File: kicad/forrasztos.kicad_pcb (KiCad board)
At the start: 2 copper layers, 115 x 70.6 mm, 91 parts, among them J1 24V+-, J2 Conn_02x04_Pin, J3 Conn_01x20_Pin, J4 Conn_01x06_Pin, J5 Conn_02x04_Pin, Q1 AOD409, Q2 MMST2222A, Q3 AOD409, Q4 MMST2222A, SW1 RotaryEncoder_Switch, SW2 SW_Push, SW3 SW_Push, U1 AP63205WU, U2 MCP6004, U3 AP63203WU, U4 24LC00, U5 STM32F103C8Tx, Y1 ATS080B

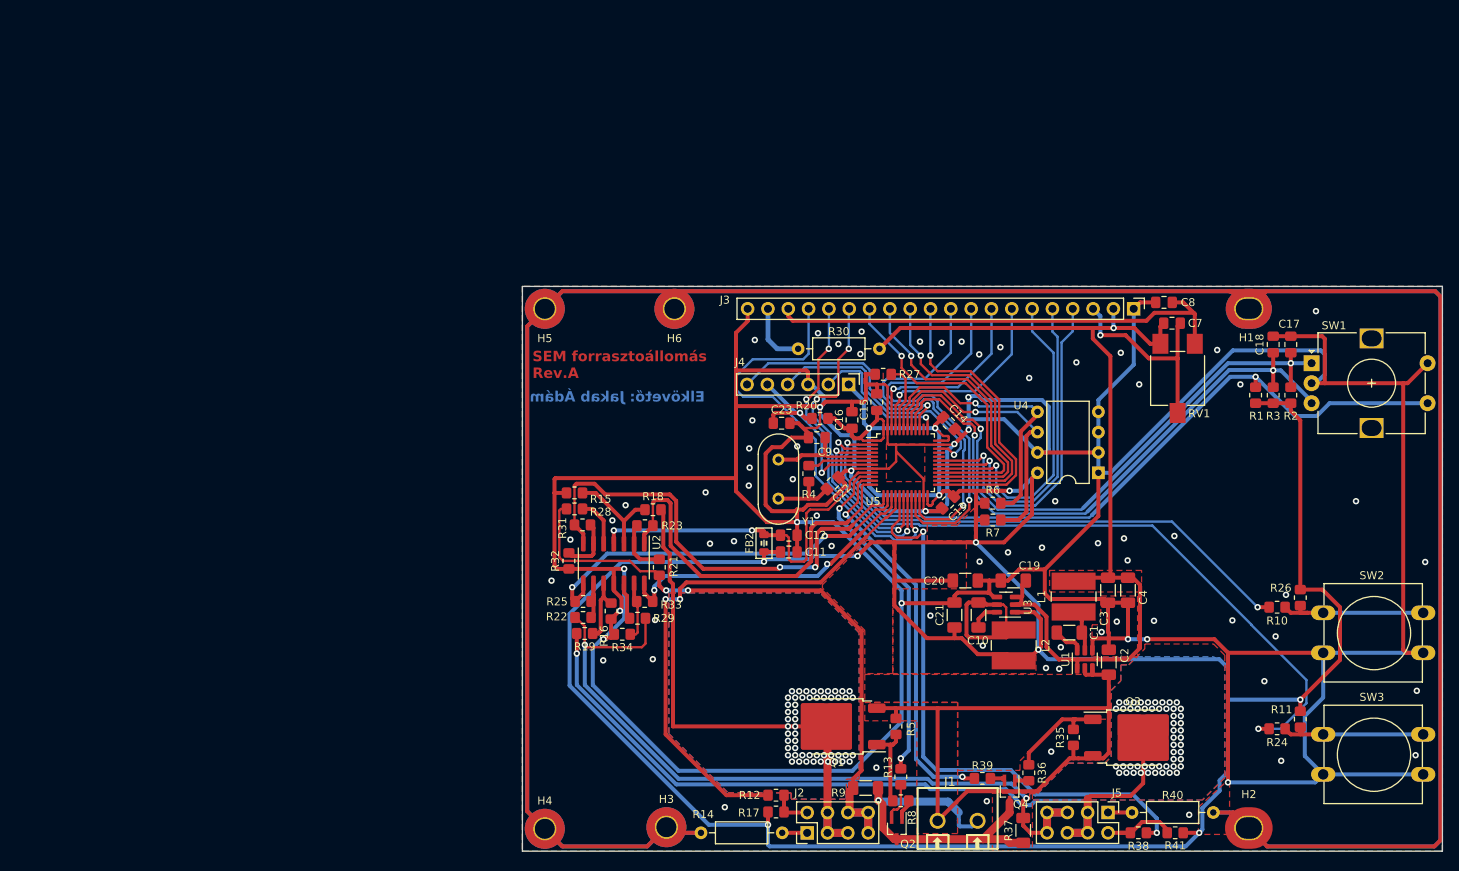
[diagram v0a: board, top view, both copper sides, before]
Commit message: hw revision
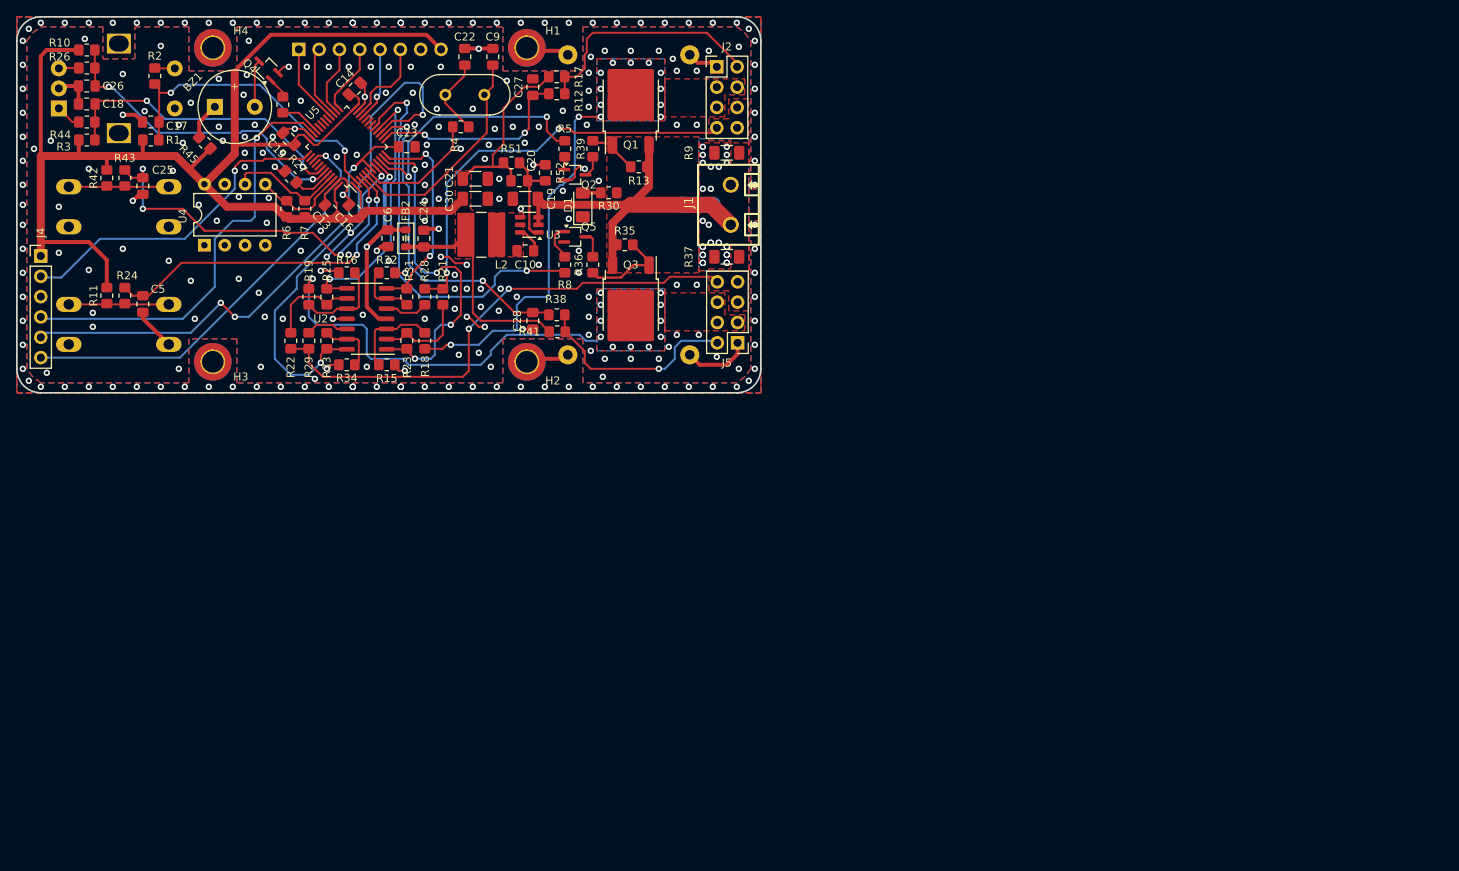
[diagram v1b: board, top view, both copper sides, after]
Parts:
- removed C1, C2: 10u, Capacitor_SMD:C_1206_3216Metric_Pad1.33x1.80mm_HandSolder
- removed C11, C12, C7, C8: 100n, Capacitor_SMD:C_0805_2012Metric_Pad1.18x1.45mm_HandSolder
- removed C3, C4: 22u, Capacitor_SMD:C_1206_3216Metric_Pad1.33x1.80mm_HandSolder
- removed the H3 at (111.2, 130.3)
- removed the H4 at (96.0, 130.5)
- removed L1: 4.7u, Inductor_SMD:L_TracoPower_TCK-047_5.2x5.8mm
- removed RV1: 10k, Potentiometer_SMD:Potentiometer_ACP_CA6-VSMD_Vertical
- removed U1: AP63205WU, Package_TO_SOT_SMD:TSOT-23-6
- added BZ1: Buzzer, forrasztos_library:BuzzerR9F5, F.Cu at (57.2, 40.2)
- added C24: 100n, Capacitor_SMD:C_0805_2012Metric_Pad1.18x1.45mm_HandSolder, F.Cu at (80.9, 56.7)
- added C25: 1u, Capacitor_SMD:C_0805_2012Metric_Pad1.18x1.45mm_HandSolder, F.Cu at (45.8, 50.1)
- added C26: 1u, Capacitor_SMD:C_0805_2012Metric_Pad1.18x1.45mm_HandSolder, F.Cu at (38.8, 37.6)
- added C27: 1u, Capacitor_SMD:C_0805_2012Metric_Pad1.18x1.45mm_HandSolder, F.Cu at (94.5, 37.8)
- added C28: 1u, Capacitor_SMD:C_0805_2012Metric_Pad1.18x1.45mm_HandSolder, F.Cu at (94.5, 67.0)
- added C30: 22u, Capacitor_SMD:C_1206_3216Metric_Pad1.33x1.80mm_HandSolder, F.Cu at (87.3, 51.8)
- added C5: 1u, Capacitor_SMD:C_0805_2012Metric_Pad1.18x1.45mm_HandSolder, F.Cu at (45.8, 64.9)
- added C6: 100n, Capacitor_SMD:C_0805_2012Metric_Pad1.18x1.45mm_HandSolder, F.Cu at (76.4, 56.7)
- added D1: LED, LED_SMD:LED_1206_3216Metric_Pad1.42x1.75mm_HandSolder, F.Cu at (100.8, 52.5)
- added Q5: SOT-23 NPN, Package_TO_SOT_SMD:SOT-323_SC-70_Handsoldering, F.Cu at (99.8, 56.5)
- added R42: 1k5, Resistor_SMD:R_0805_2012Metric_Pad1.20x1.40mm_HandSolder, F.Cu at (41.2, 49.1)
- added R43: 4k7, Resistor_SMD:R_0805_2012Metric_Pad1.20x1.40mm_HandSolder, F.Cu at (43.5, 49.1)
- added R44: 4k7, Resistor_SMD:R_0805_2012Metric_Pad1.20x1.40mm_HandSolder, F.Cu at (38.8, 42.1)
- added R45: 150, Resistor_SMD:R_0805_2012Metric_Pad1.20x1.40mm_HandSolder, F.Cu at (53.5, 44.8)
- added R51: 182k, Resistor_SMD:R_0805_2012Metric_Pad1.20x1.40mm_HandSolder, F.Cu at (91.8, 47.2)
- added R52: 62k, Resistor_SMD:R_0805_2012Metric_Pad1.20x1.40mm_HandSolder, F.Cu at (96.1, 48.5)
- C10: value 10u -> 100n; footprint Capacitor_SMD:C_1206_3216Metric_Pad1.33x1.80mm_HandSolder -> Capacitor_SMD:C_0805_2012Metric_Pad1.18x1.45mm_HandSolder
- C17, C18: value 1n -> 1u
- C20: value 22u -> 100p; footprint Capacitor_SMD:C_1206_3216Metric_Pad1.33x1.80mm_HandSolder -> Capacitor_SMD:C_0805_2012Metric_Pad1.18x1.45mm_HandSolder
- H1: footprint forrasztos_library:MountingHoleOval_3.27x2.5mm -> MountingHole:MountingHole_2.7mm_M2.5_DIN965_Pad_TopBottom
- H2: footprint forrasztos_library:MountingHoleOval_3.27x2.7mm -> MountingHole:MountingHole_2.7mm_M2.5_DIN965_Pad_TopBottom
- H3: renamed from H5; footprint MountingHole:MountingHole_2.5mm_Pad_TopBottom -> MountingHole:MountingHole_2.7mm_M2.5_DIN965_Pad_TopBottom
- H4: renamed from H6; footprint MountingHole:MountingHole_2.5mm_Pad_TopBottom -> MountingHole:MountingHole_2.7mm_M2.5_DIN965_Pad_TopBottom
- J3: value Conn_01x20_Pin -> Conn_01x08_Pin; footprint Connector_PinHeader_2.54mm:PinHeader_1x20_P2.54mm_Vertical -> Connector_PinHeader_2.54mm:PinHeader_1x08_P2.54mm_Vertical; moved to B.Cu
- L2: value 4.7u -> 6.8u
- NT1: footprint NetTie:NetTie-2_SMD_Pad0.5mm -> NetTie:NetTie-2_SMD_Pad2.0mm
- Q1, Q3: value AOD409 -> DPAK PMOS
- Q2: value MMST2222A -> SOT-23 NPN
- Q4: value MMST2222A -> MMBT2222A
- R1, R11, R17, R3, R41: value 10k -> 1k5
- R10: value 1k -> 1k5
- R12, R24, R38: value 1k -> 4k7
- R13, R35: value 1k -> 470
- R14, R40: value 100k -> 1M; footprint Resistor_THT:R_Axial_DIN0207_L6.3mm_D2.5mm_P10.16mm_Horizontal -> Resistor_THT:R_Axial_DIN0414_L11.9mm_D4.5mm_P15.24mm_Horizontal; moved to B.Cu
- R15, R16, R23, R25: value 1.5M -> 1M5
- R2, R26: value 10k -> 4k7
- R20: value 10k -> 1k
- R30: value 50 -> 1k5; footprint Resistor_THT:R_Axial_DIN0207_L6.3mm_D2.5mm_P10.16mm_Horizontal -> Resistor_SMD:R_0805_2012Metric_Pad1.20x1.40mm_HandSolder
- SW1, SW2, SW3: moved to B.Cu
- moved R26 165.5 mm to (38.8, 35.4), turned to 0 degrees
- moved R10 164.3 mm to (38.8, 33.1), turned to 180 degrees
- moved SW1 159.8 mm to (35.2, 40.5)
- moved R11 158.3 mm to (41.2, 63.9)
- moved SW3 154.0 mm to (49.0, 65.0), turned to 180 degrees
- moved R24 153.9 mm to (43.5, 63.9), turned to -90 degrees
- moved SW2 153.8 mm to (49.0, 50.2), turned to 180 degrees
- moved R3 151.7 mm to (38.8, 44.4), turned to 180 degrees
- moved C18 151.3 mm to (38.8, 39.9), turned to 180 degrees
- moved R2 147.5 mm to (47.2, 36.4), turned to -90 degrees
- moved C17 145.2 mm to (46.8, 42.1), turned to 180 degrees
- moved R1 141.7 mm to (46.8, 44.4), turned to 180 degrees
- moved Q4 129.5 mm to (61.2, 35.5), turned to 135 degrees
- moved U4 115.3 mm to (53.5, 57.5), turned to 90 degrees
- moved J3 109.3 mm to (65.2, 33.1)
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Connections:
- net /CRYSTAL_1 renamed /CRYSTAL_IN
- net /CRYSTAL_2 renamed /CRYSTAL_OUT
- C17 pad 1: /ENC_B -> /ENC_SW
- C19 pad 1: +5V -> +24V
- C20 pad 2: GND -> Net-(U3-FB)
- C23 pad 1: /NRST -> GND
- C23 pad 2: GND -> /NRST
- H1 pad 1: GND -> Earth_Protective
- H2 pad 1: GND -> Earth_Protective
- H3 pad 1: GND -> Earth_Protective
- H4 pad 1: GND -> Earth_Protective
- J1 pad 2: GND -> GNDPWR
- J3 pad 1: GND -> /LCD_BL
- J3 pad 2: +5V -> /LCD_CLK
- J3 pad 3: /LCD_V0 -> /LCD_DIN
- J3 pad 4: /LCD_DI -> /LCD_DC
- J3 pad 5: /LCD_RW -> /LCD_RST
- J3 pad 6: /LCD_E -> /LCD_CE
- J3 pad 7: /LCD_D0 -> GND
- J3 pad 8: /LCD_D1 -> +3.3V
- Q2 pad 1: Net-(Q2-C) -> Net-(Q2-B)
- Q2 pad 2: Net-(Q2-B) -> GND
- Q2 pad 3: GNDPWR -> Net-(Q2-C)
- Q4 pad 1: Net-(Q4-C) -> Net-(Q4-B)
- Q4 pad 2: Net-(Q4-B) -> GND
- Q4 pad 3: GNDPWR -> Net-(BZ1--)
- R1 pad 1: +3.3V -> /ENC_SW
- R1 pad 2: /ENC_SW -> +3.3V
- R10 pad 1: /BTN_1 -> /ENC_B
- R10 pad 2: Net-(R10-Pad2) -> +3.3V
- R13 pad 1: Net-(Q2-B) -> Net-(Q1-G)
- R13 pad 2: /CH1_HEATER -> +24V
- R14 pad 1: GND -> Earth_Protective
- R17 pad 1: Net-(J2-Pin_4) -> +3.3V
- R17 pad 2: +3.3V -> Net-(J2-Pin_4)
- R2 pad 1: +3.3V -> Net-(R2-Pad1)
- R2 pad 2: /ENC_B -> /ENC_SW
- R20 pad 1: /NRST -> Net-(Q4-B)
- R20 pad 2: +3.3V -> /BUZZER
- R21 pad 1: /CH1_AMP_N -> Net-(U2A--)
- R21 pad 2: Net-(U2A--) -> /CH1_AMP_N
- R22 pad 1: /CH2_AMP_N -> Net-(U2C--)
- R22 pad 2: Net-(U2C--) -> /CH2_AMP_N
- R26 pad 1: Net-(R10-Pad2) -> Net-(R26-Pad1)
- R26 pad 2: +3.3V -> /ENC_B
- R3 pad 1: +3.3V -> /ENC_A
- R3 pad 2: /ENC_A -> +3.3V
- R30 pad 1: +5V -> +24V
- R30 pad 2: Net-(J3-Pin_19) -> Net-(D1-A)
- R36 pad 2: Net-(Q4-C) -> Net-(Q5-C)
- R39 pad 1: Net-(Q4-B) -> Net-(Q2-C)
- R39 pad 2: /CH2_HEATER -> Net-(Q1-G)
- R40 pad 1: GND -> Earth_Protective
- R5 pad 1: +24V -> Net-(Q2-B)
- R5 pad 2: Net-(Q1-G) -> /CH1_HEATER
- R8 pad 1: Net-(Q1-G) -> Net-(Q5-B)
- R8 pad 2: Net-(Q2-C) -> /CH2_HEATER
- SW1 pad A: /ENC_B -> Net-(R44-Pad1)
- SW1 pad B: /ENC_A -> Net-(R26-Pad1)
- SW1 pad S2: /ENC_SW -> Net-(R2-Pad1)
- SW2 pad 1: Net-(R10-Pad2) -> Net-(R42-Pad1)
- U3 pad 1: +3.3V -> Net-(U3-FB)
- U3 pad 2: +5V -> +24V
- U3 pad 3: +5V -> +24V
- U5 pad 11: /CH2_HEATER -> /CH1_THERMO
- U5 pad 12: /CH1_THERMO -> /CH1_CURRENT
- U5 pad 13: /CH1_CURRENT -> /CH1_TILT
- U5 pad 14: /CH2_THERMO -> /CH2_TILT
- U5 pad 16: /CH1_TILT -> /CH2_THERMO
- U5 pad 17: /CH2_TILT -> /CH2_HEATER
- U5 pad 18: /LCD_CS1 -> unconnected-(U5-PB0-Pad18)
- U5 pad 19: /LCD_CS2 -> unconnected-(U5-PB1-Pad19)
- U5 pad 20: /LCD_RST -> unconnected-(U5-PB2-Pad20)
- U5 pad 21: /LCD_D2 -> /LCD_RST
- U5 pad 22: /LCD_D3 -> /LCD_CE
- U5 pad 25: /LCD_D4 -> /LCD_DC
- U5 pad 26: /LCD_D5 -> /LCD_DIN
- U5 pad 27: /LCD_D6 -> /LCD_CLK
- U5 pad 28: /LCD_D7 -> /LCD_BL
- U5 pad 29: /LCD_E -> unconnected-(U5-PA8-Pad29)
- U5 pad 30: /LCD_RW -> unconnected-(U5-PA9-Pad30)
- U5 pad 31: /LCD_DI -> unconnected-(U5-PA10-Pad31)
- U5 pad 33: unconnected-(U5-PA12-Pad33) -> /BUZZER
- U5 pad 40: /ENC_A -> unconnected-(U5-PB4-Pad40)
- U5 pad 41: /ENC_B -> unconnected-(U5-PB5-Pad41)
- U5 pad 42: /i2c_SCL -> /ENC_A
- U5 pad 43: /i2c_SDA -> /ENC_B
- U5 pad 45: /LCD_D0 -> /i2c_SCL
- U5 pad 46: /LCD_D1 -> /i2c_SDA
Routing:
- net GND: track 1286.5 -> 77.4 mm, vias 79 -> 162
- net +3.3V: track 428.1 -> 237.3 mm, vias 11 -> 0
- net +5V: track 117.9 -> 0.00 mm, vias 1 -> 0
- net /LCD_VOUT: track 59.6 -> 0.00 mm
- net /ENC_SW: track 93.8 -> 39.2 mm
- net /CH2_AMP_P: track 103.2 -> 49.7 mm, vias 53 -> 12
- net /LCD_D2: track 51.4 -> 0.00 mm, vias 1 -> 0
- net /LCD_D3: track 47.7 -> 0.00 mm, vias 1 -> 0
- net /LCD_RST: track 55.8 -> 9.22 mm
- net /BTN_2: track 88.9 -> 42.9 mm
- net /LCD_DI: track 43.8 -> 0.00 mm, vias 1 -> 0
- net /CH1_TILT: track 68.7 -> 25.5 mm
- net /LCD_RW: track 41.6 -> 0.00 mm, vias 1 -> 0
- net /LCD_CS2: track 41.5 -> 0.00 mm, vias 3 -> 0
- net /LCD_CS1: track 41.0 -> 0.00 mm, vias 3 -> 0
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- added copper zone on F.Cu, net /CH1_AMP_N
- added copper zone on F.Cu, net /CH2_AMP_N
- added copper zone on B.Cu, net Earth_Protective
- added copper zone on F.Cu, net Earth_Protective
- added copper zone on B.Cu, net GNDPWR
- added copper zone on F.Cu, net Net-(U3-SW)
- removed copper zone on B.Cu, net +3.3V
- removed copper zone on F.Cu, net +5V
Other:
- board size 115 x 70.6 mm -> 93 x 47 mm
- rule pad_to_mask_clearance: 0 -> 0.038
- board text added: "SEM forrasztóállomás Rev.B Elkövető: J. Á."
- board text removed: "Elkövető: Jakab Ádám"
- board text removed: "SEM forrasztoállomás Rev.A"
